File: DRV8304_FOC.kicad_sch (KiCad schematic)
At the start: 64 parts, among them J1 Conn_01x02, J2 Conn_01x03, J3 Conn_01x03, Q1 SIRA18ADP, Q2 SIRA18ADP, Q3 SIRA18ADP, Q4 SIRA18ADP, Q5 SIRA18ADP, Q6 SIRA18ADP, SW2 SW_Push, U1 TPS565208, U2 TPS259850RQPR, U3 DRV8304HRHAR, U4 STM32F412CEUx, U5 AS5055A, Y1 Crystal_GND23

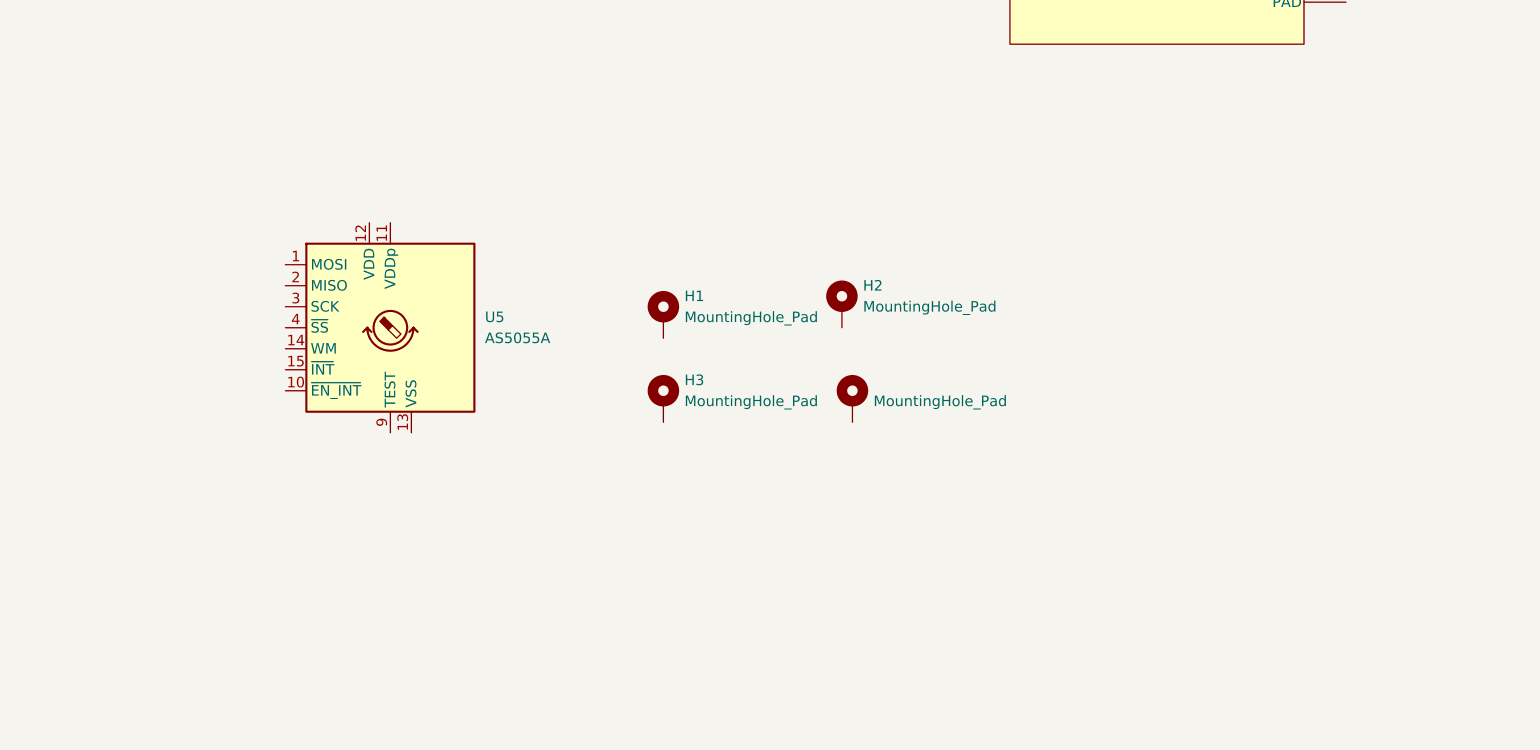
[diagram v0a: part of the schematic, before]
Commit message: hall sensor
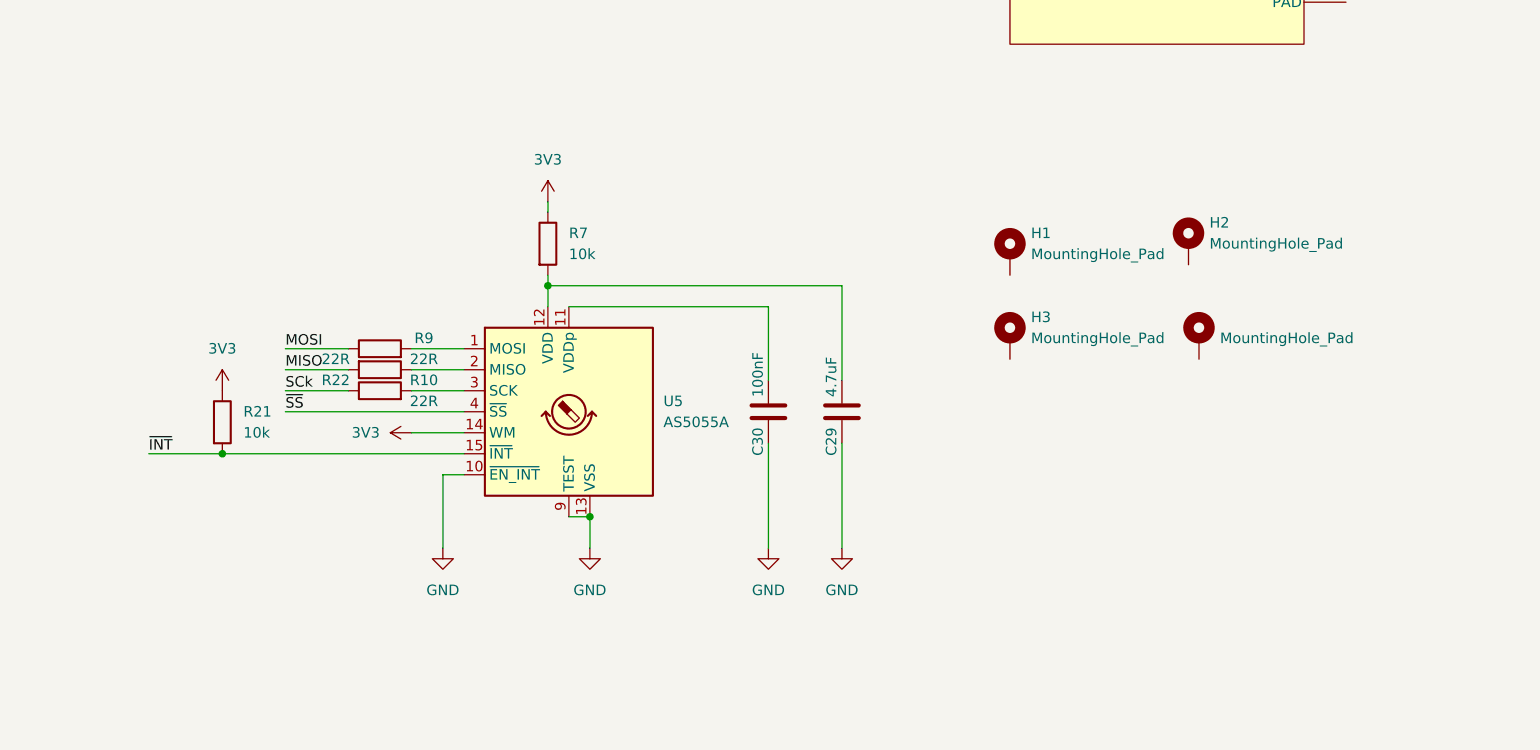
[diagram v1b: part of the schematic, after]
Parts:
- added C29: 4.7uF, Capacitor_SMD:C_0603_1608Metric, symbol Device:C
- added C30: 100nF, Capacitor_SMD:C_0402_1005Metric, symbol Device:C
- added R10, R22, R9: 22R, Resistor_SMD:R_0402_1005Metric, symbol Device:R
- added R21, R7: 10k, Resistor_SMD:R_0402_1005Metric, symbol Device:R
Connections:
- net 3V3: now also U5.14 (WM), R21.1, R7.1
- net GND: now also U5.10 (~{EN_INT}), U5.13 (VSS), U5.9 (TEST), C29.2, C30.2
- net at U5.1 (MOSI): now also R9.2
- net at U5.11 (VDDp): now also C30.1
- net at U5.12 (VDD): now also C29.1, R7.2
- net ~{INT}: now reaches U5.15 (~{INT})
- net ~{INT}: now also R21.2
- net at U5.2 (MISO): now also R22.1
- net at U5.3 (SCK): now also R10.2
- net ~{SS}: now reaches U5.4 (~{SS})
- new net MISO: R22.2
- new net MOSI: R9.1
- new net SCk: R10.1
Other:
- moved on the sheet: H1, H2, H3
